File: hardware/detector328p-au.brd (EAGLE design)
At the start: 40 x 70 mm, 67 parts, among them K1 SRD-05VDC-SL-C, Q1 BSS123, Q2 16MHz, T1 BC817-40SMD, T2 BC817, T3 BC817, U1 ATMEGA328P-AU

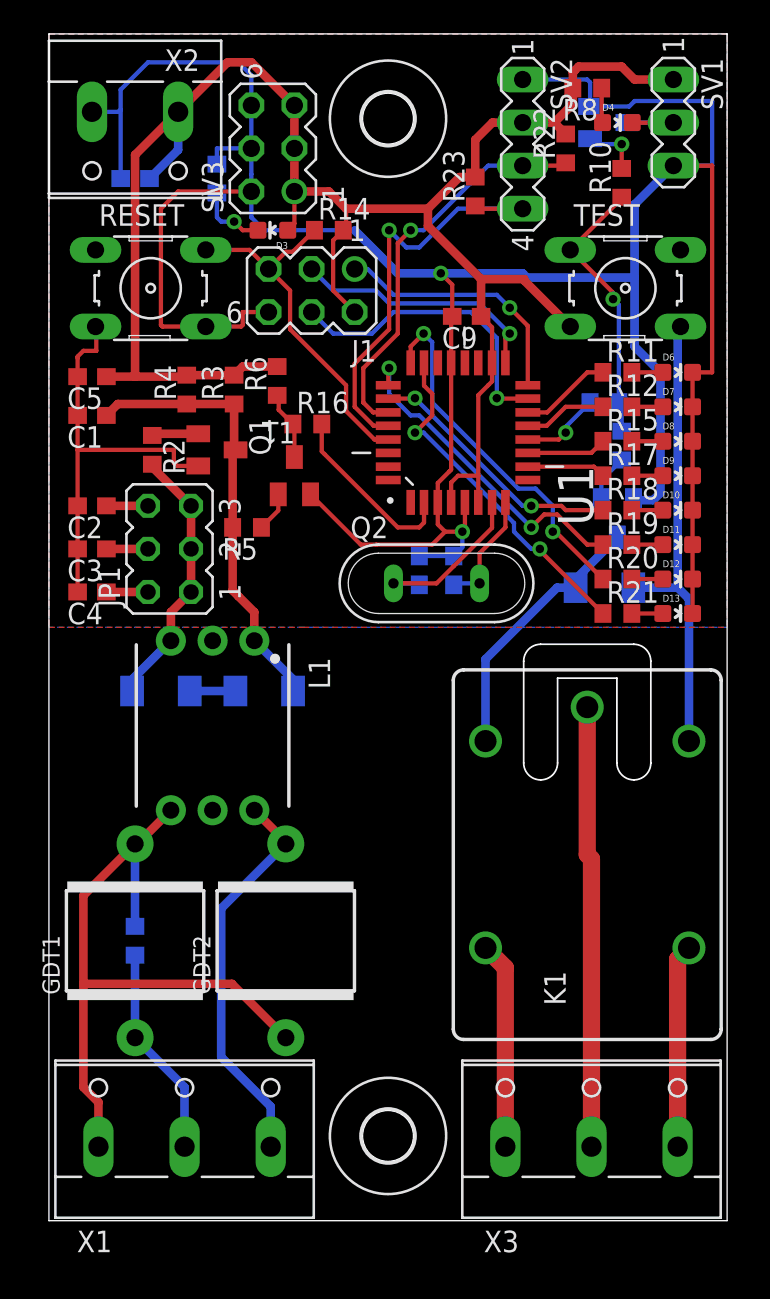
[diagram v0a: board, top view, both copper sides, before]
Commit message: detector328p-au final
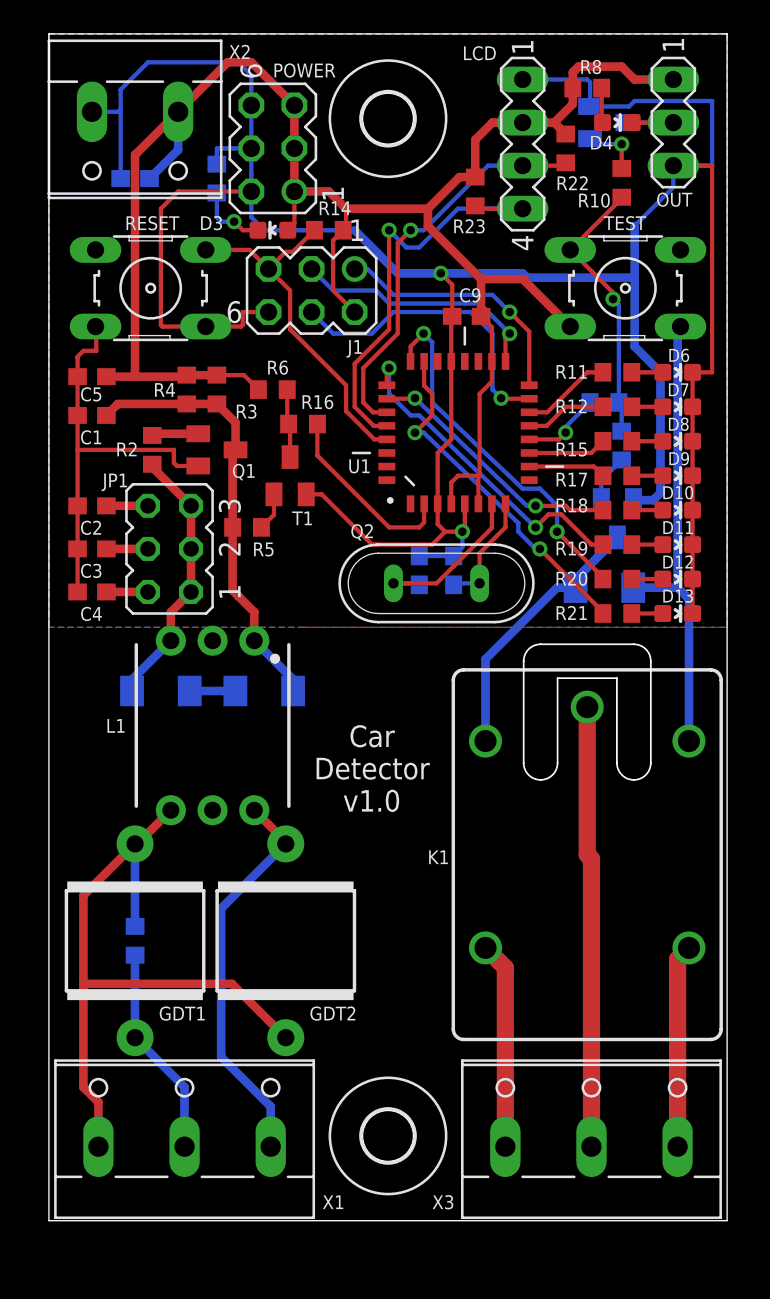
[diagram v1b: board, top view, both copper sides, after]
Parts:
- moved R3 1.02 mm to (9.91, 49.0)
- moved R6 0.57 mm to (13.2, 49.0), turned to 180 degrees
- moved R16 0.25 mm to (15.0, 47.0)
- moved T1 0.25 mm to (14.2, 43.9)
- renumbered SV1 to OUT, SV2 to LCD, SV3 to POWER
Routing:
- net VCC: track 141.2 -> 140.5 mm
- net GND: track 198.8 -> 199.4 mm
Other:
- board text added: "Car Detector v1.0"
